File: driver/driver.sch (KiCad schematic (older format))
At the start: 24 parts, among them J1 Screw_Terminal_01x04, J2 Screw_Terminal_01x04, J3 Conn_01x03_Female, J4 Conn_01x03_Female, J5 Barrel_Jack, SW1 SW_SPDT, SW2 SW_SPDT, SW3 SW_SPDT, U1 NCP1117ST50T3G

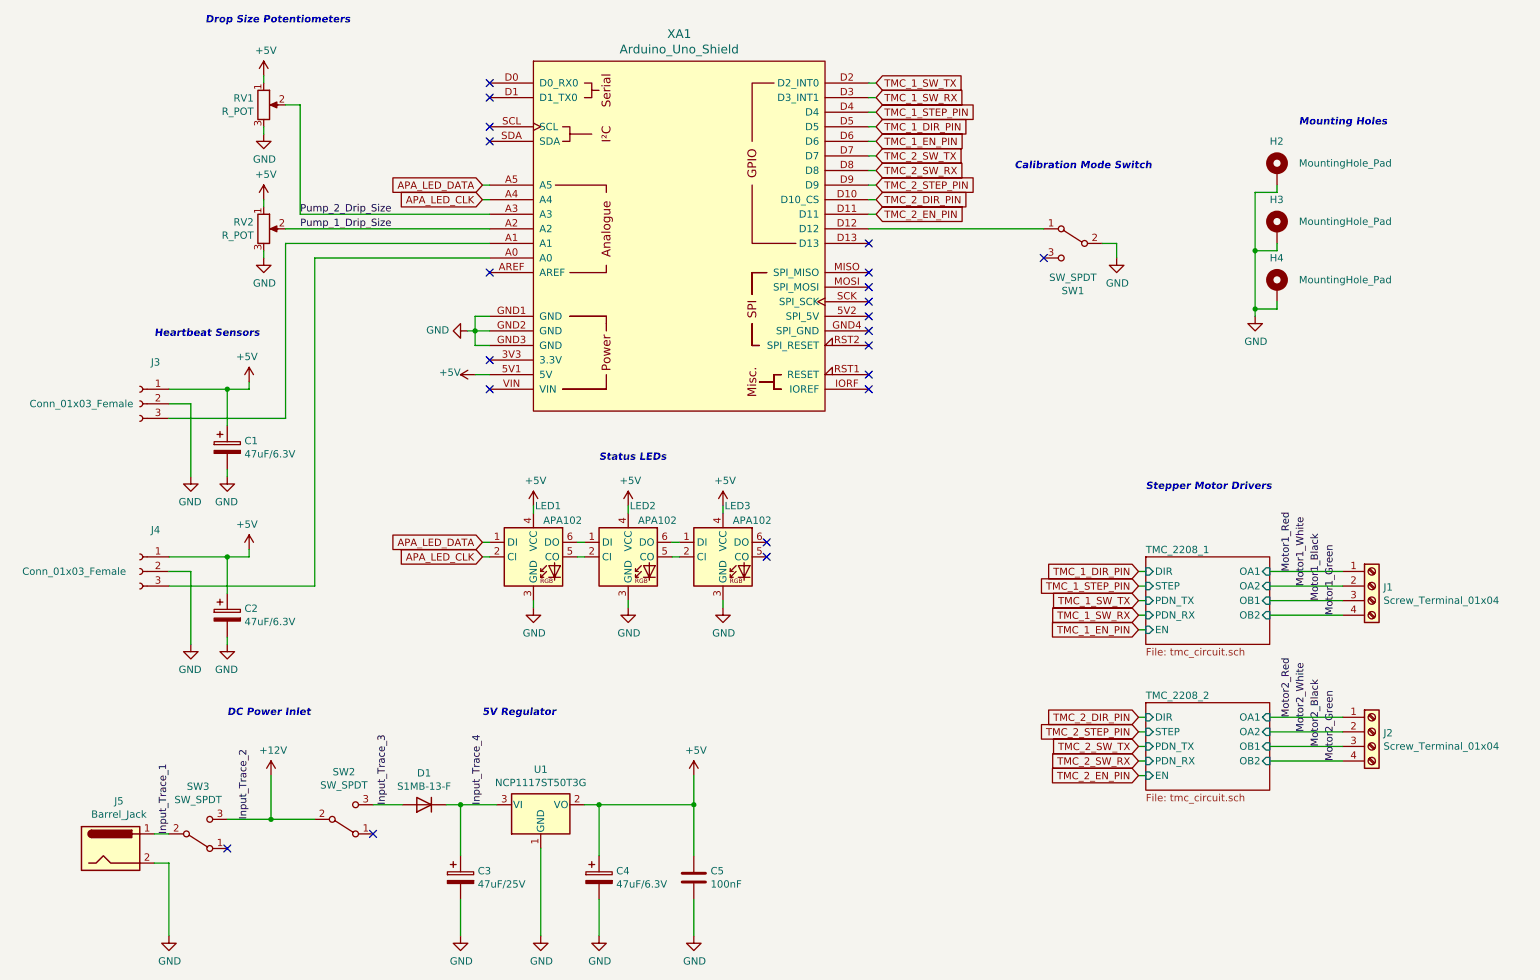
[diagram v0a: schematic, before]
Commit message: Design is finished, ordering boards
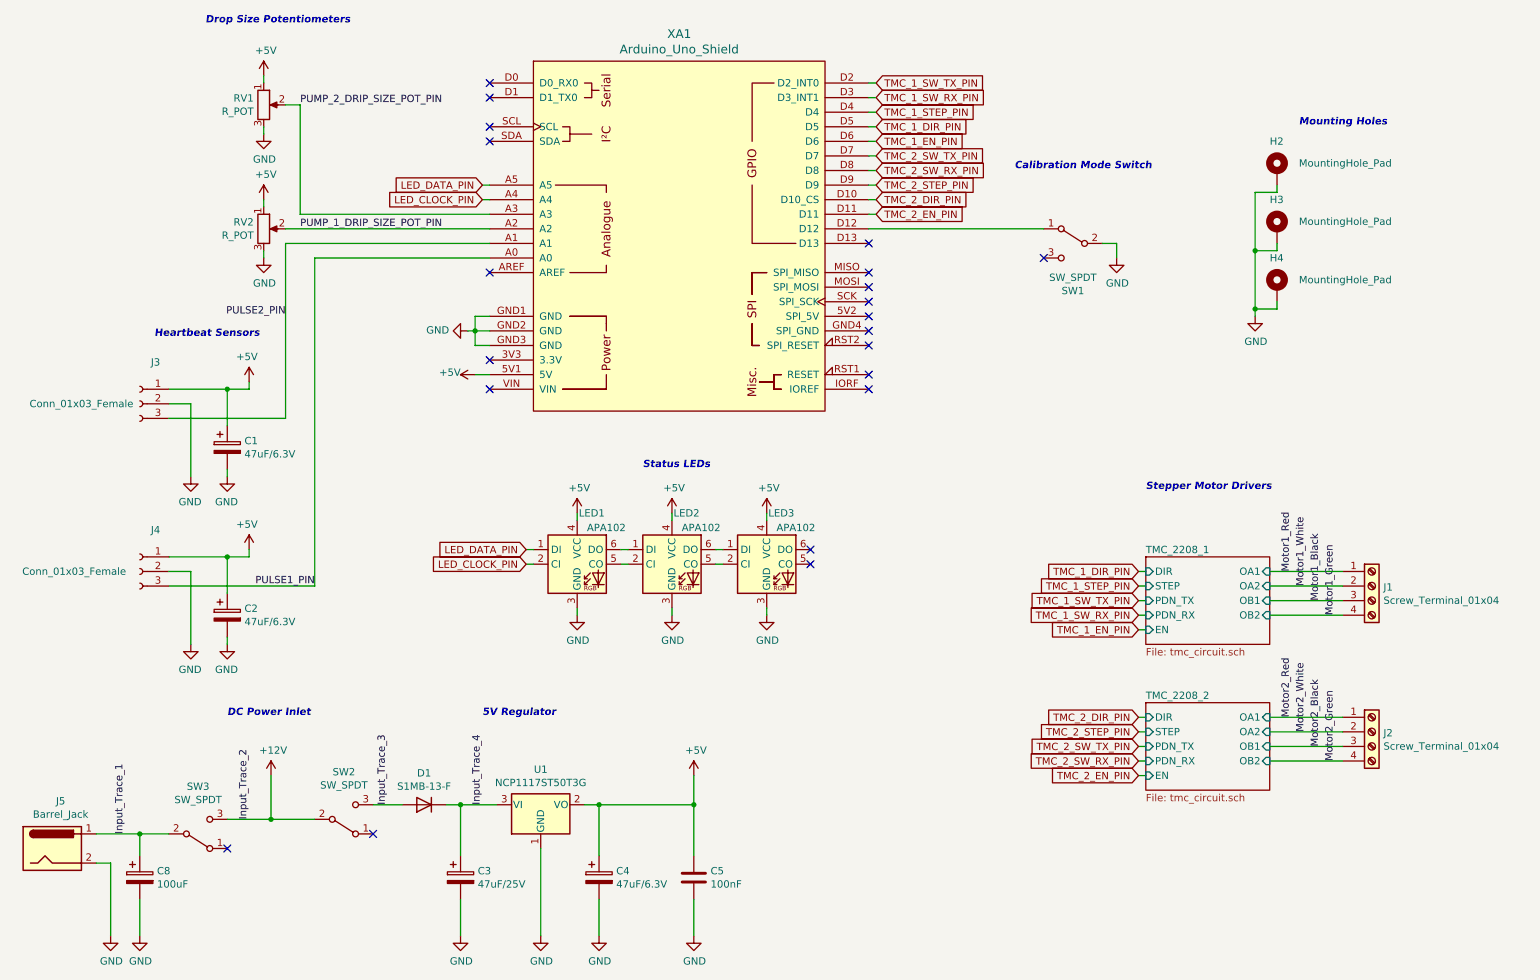
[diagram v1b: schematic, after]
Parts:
- added C8: 100uF, Capacitor_SMD:CP_Elec_6.3x5.8, symbol Device:CP
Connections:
- net GND: now also C8.2
- net Input_Trace_1: now also C8.1
- net PULSE1_PIN: now reaches J4.3 (Pin_3), XA1.A0
- net PULSE2_PIN: now reaches J3.3 (Pin_3), XA1.A1
- net APA_LED_CLK renamed LED_CLOCK_PIN
- net APA_LED_DATA renamed LED_DATA_PIN
- net Pump_1_Drip_Size renamed PUMP_1_DRIP_SIZE_POT_PIN
- net Pump_2_Drip_Size renamed PUMP_2_DRIP_SIZE_POT_PIN
- net TMC_1_SW_RX renamed TMC_1_SW_RX_PIN
- net TMC_1_SW_TX renamed TMC_1_SW_TX_PIN
- net TMC_2_SW_RX renamed TMC_2_SW_RX_PIN
- net TMC_2_SW_TX renamed TMC_2_SW_TX_PIN
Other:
- moved on the sheet: J5, LED1, LED2, LED3
